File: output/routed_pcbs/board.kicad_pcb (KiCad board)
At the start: 2 copper layers, 122.3 x 101.1 mm, 39 parts

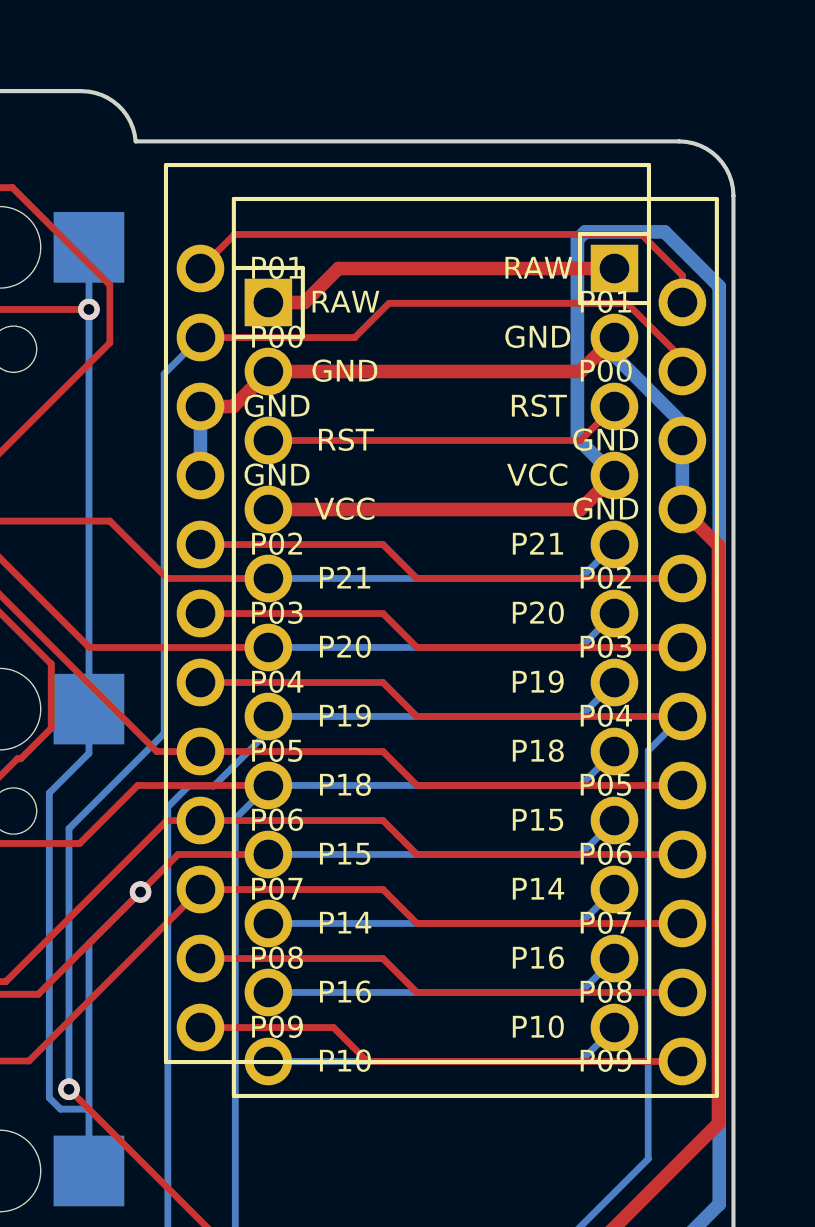
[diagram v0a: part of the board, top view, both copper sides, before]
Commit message: A probably working version
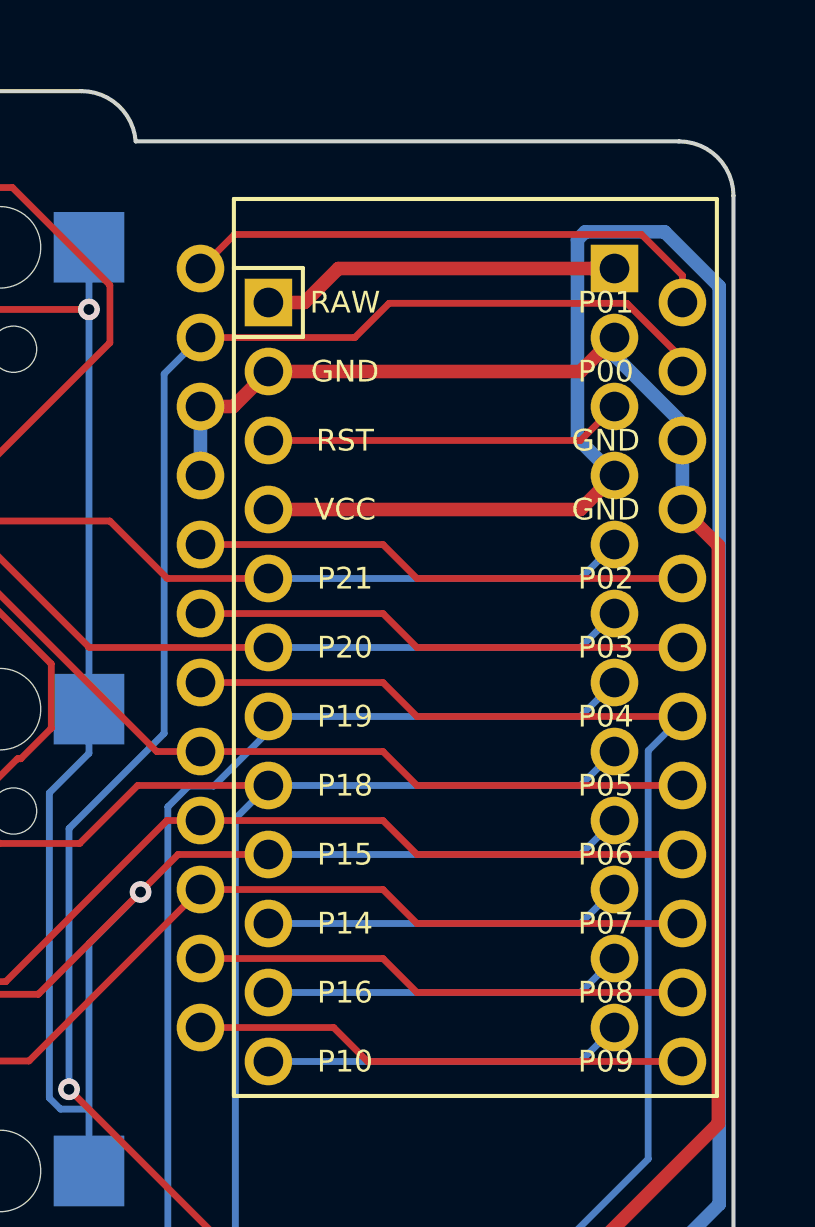
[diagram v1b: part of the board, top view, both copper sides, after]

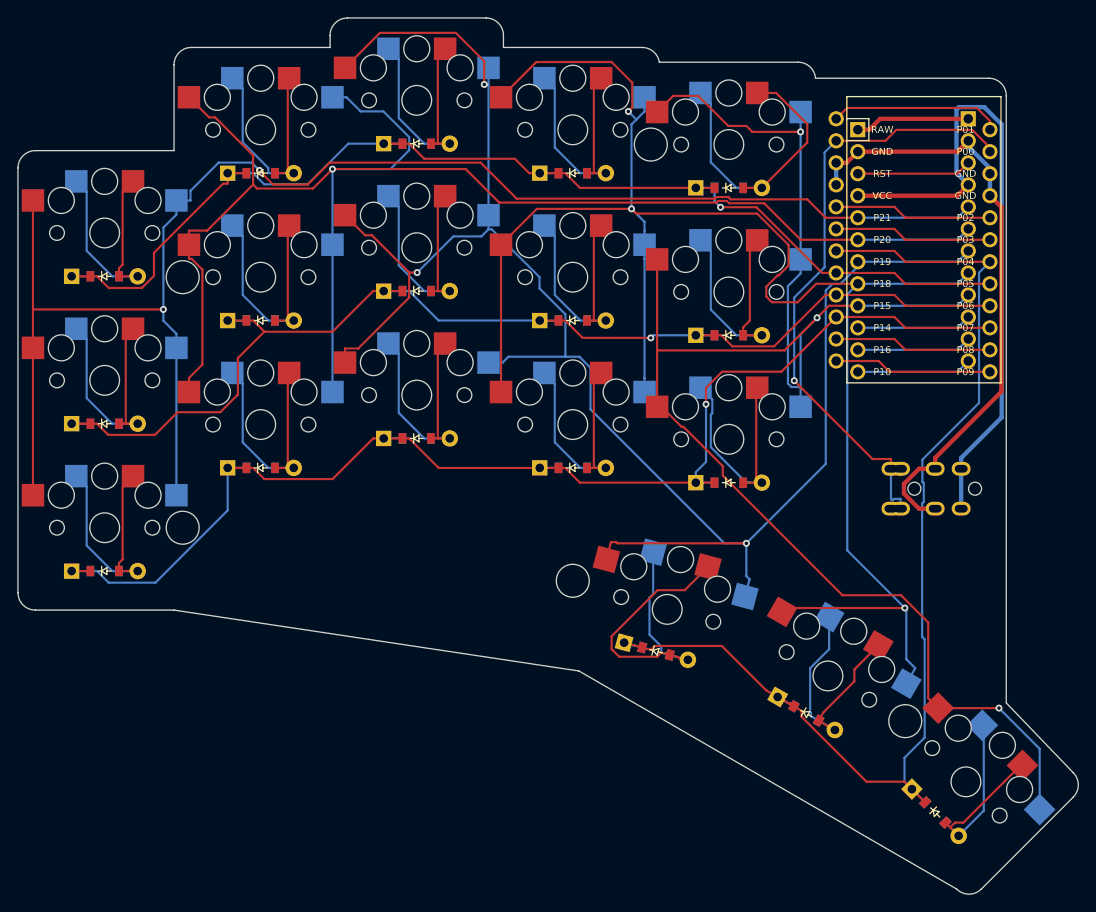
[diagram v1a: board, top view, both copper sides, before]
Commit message: Add output files
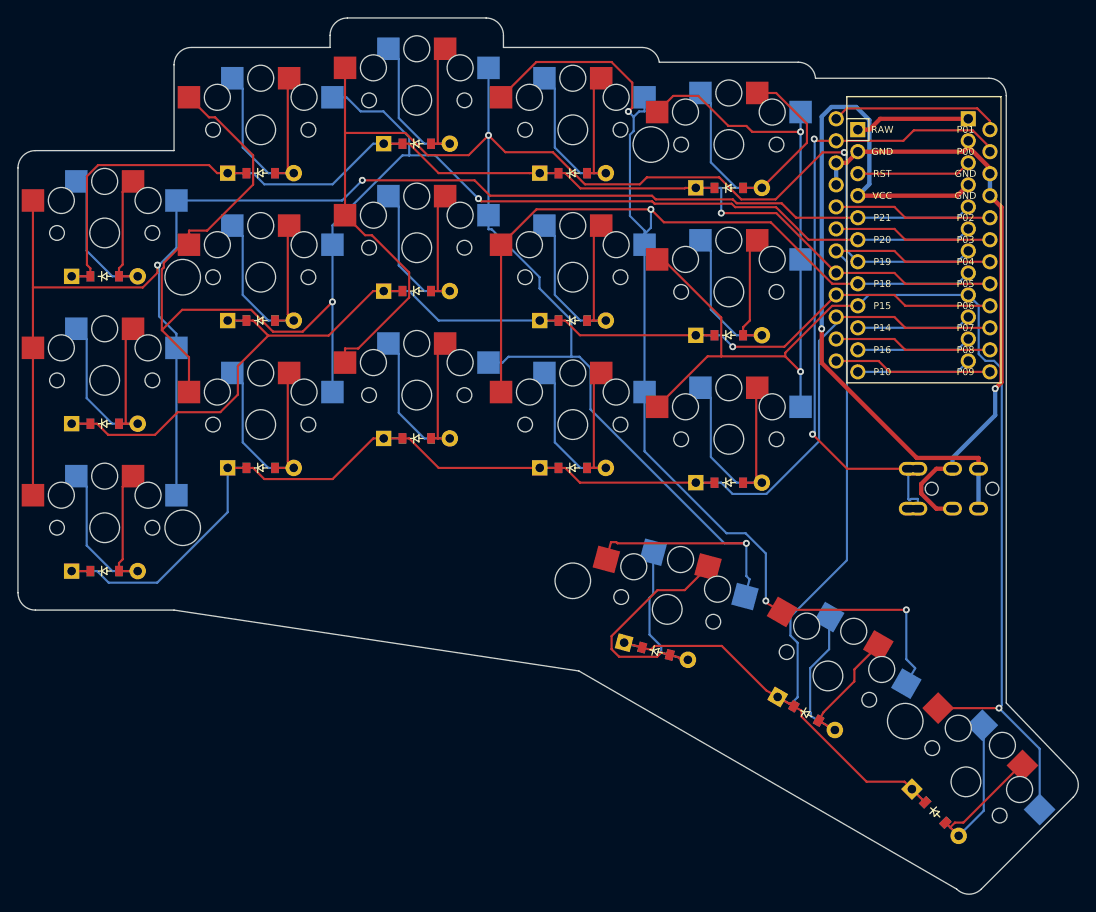
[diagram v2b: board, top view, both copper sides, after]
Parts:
- moved REF** 2.00 mm to (122.0, -2.20)
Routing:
- net P19: track 212.6 -> 236.9 mm
- net P18: track 208.0 -> 194.9 mm, vias 3 -> 4
- net VCC: track 74.9 -> 86.0 mm, vias 0 -> 1
- net P15: track 192.6 -> 182.3 mm
- net P4: track 133.2 -> 123.6 mm
- net P5: track 135.1 -> 140.7 mm
- net P0: track 73.3 -> 77.0 mm, vias 1 -> 2
- net P21: track 183.5 -> 180.4 mm
- net P20: track 178.6 -> 181.6 mm, vias 1 -> 2
- net GND: track 71.2 -> 70.1 mm, vias 0 -> 1
- net P7: track 146.5 -> 147.1 mm, vias 1 -> 0
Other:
- outline, holes or cut-outs redrawn
